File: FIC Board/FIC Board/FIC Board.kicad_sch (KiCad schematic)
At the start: 0 parts

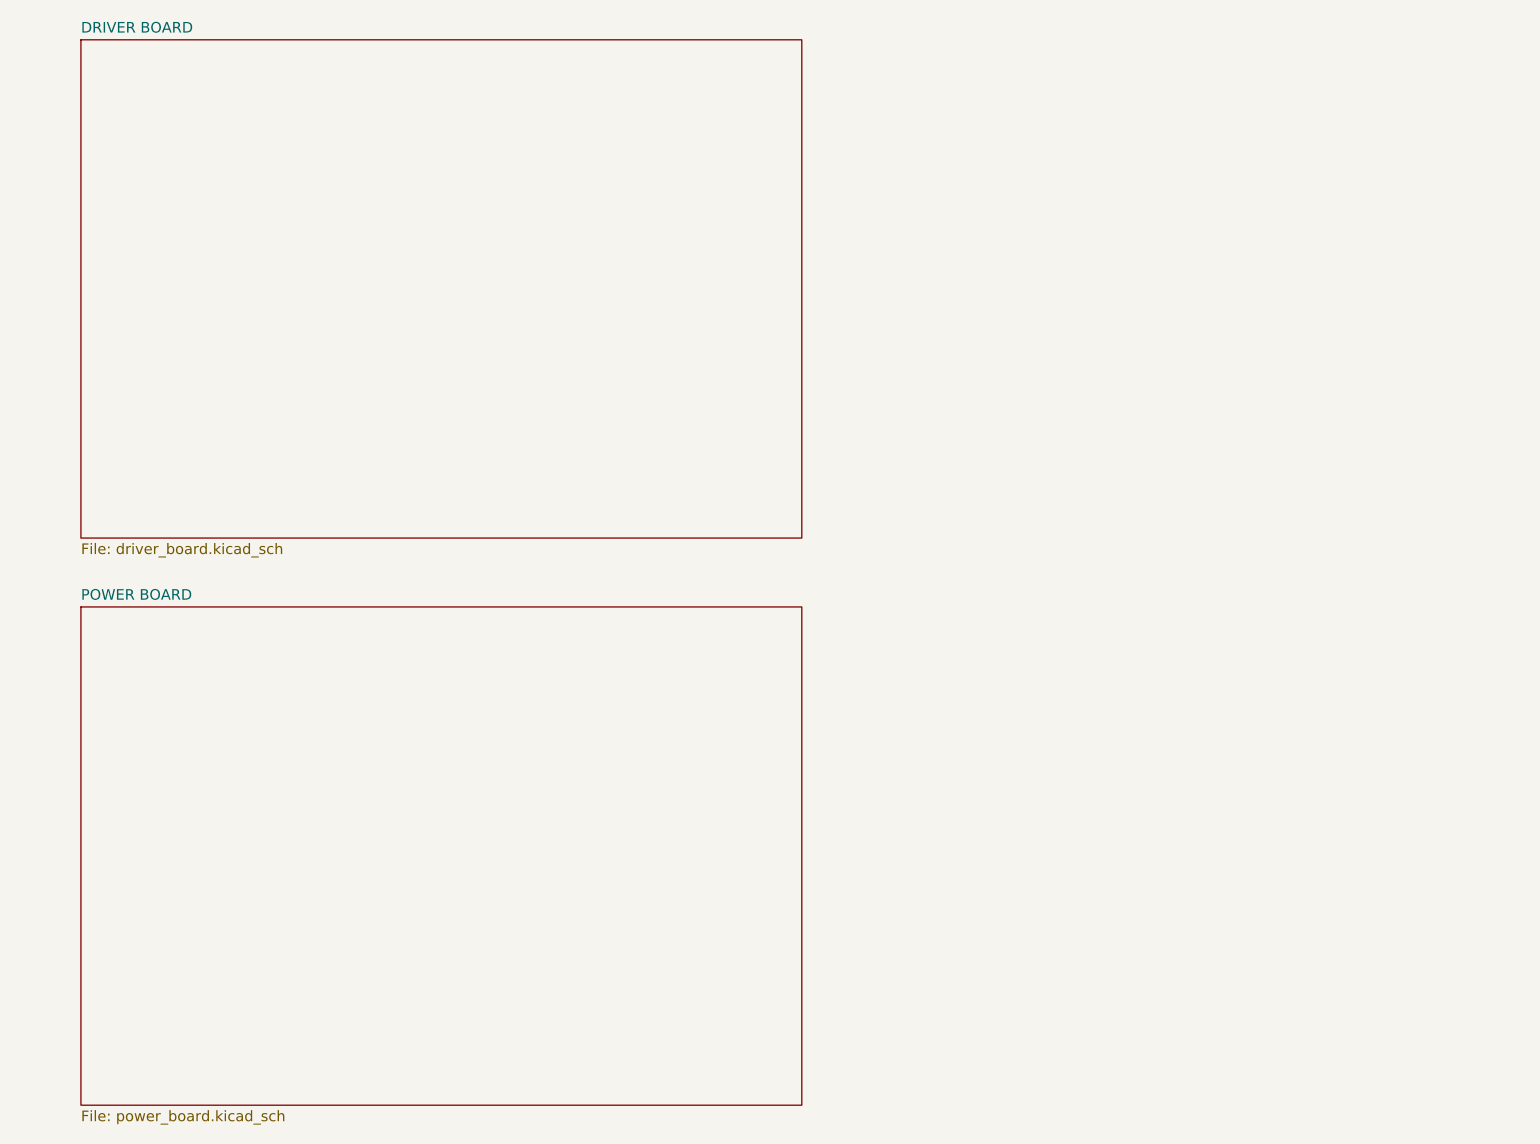
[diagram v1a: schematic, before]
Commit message: recent
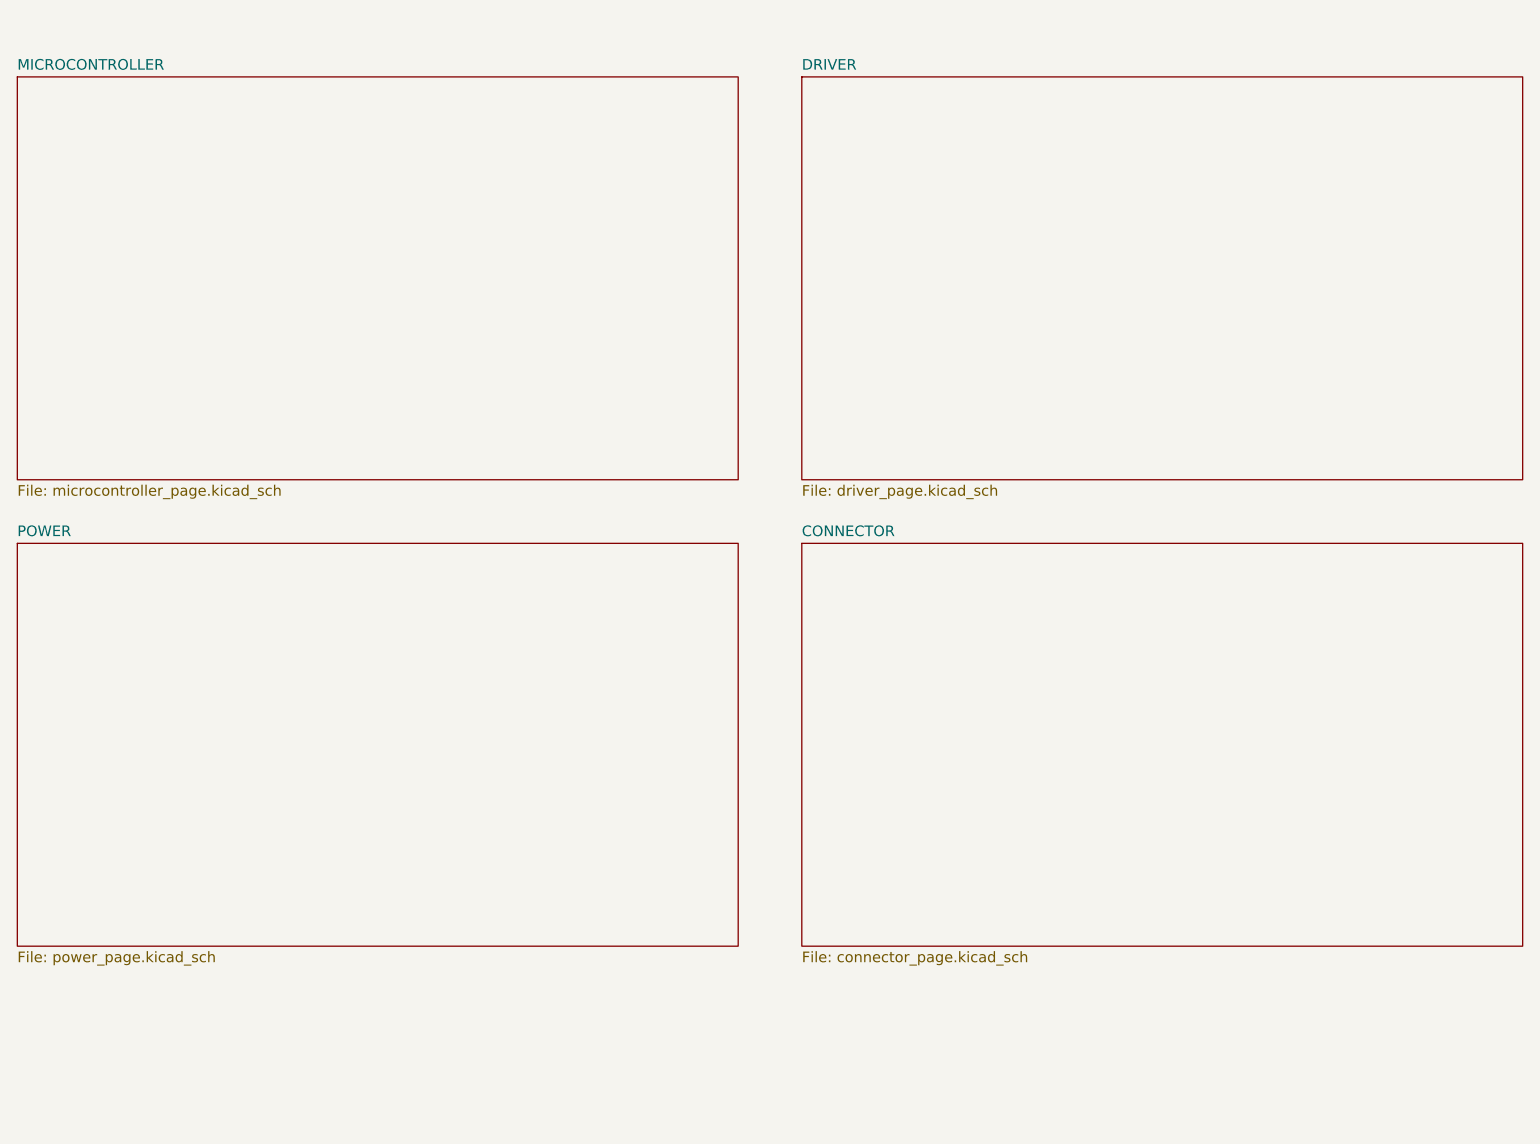
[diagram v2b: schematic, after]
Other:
- sheet DRIVER BOARD renamed MICROCONTROLLER
- sheet POWER BOARD renamed POWER
- added sheet CONNECTOR (connector_page.kicad_sch)
- added sheet DRIVER (driver_page.kicad_sch)
- sheet MICROCONTROLLER: file driver_board.kicad_sch -> microcontroller_page.kicad_sch
- sheet POWER: file power_board.kicad_sch -> power_page.kicad_sch
